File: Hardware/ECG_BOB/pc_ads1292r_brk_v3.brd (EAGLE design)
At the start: 33.9 x 39.9 mm, 64 parts, among them Q1 BSS138, Q2 BSS138, Q3 BSS138, Q4 BSS138, Q5 BSS138, Q6 BSS138, Q7 BSS138

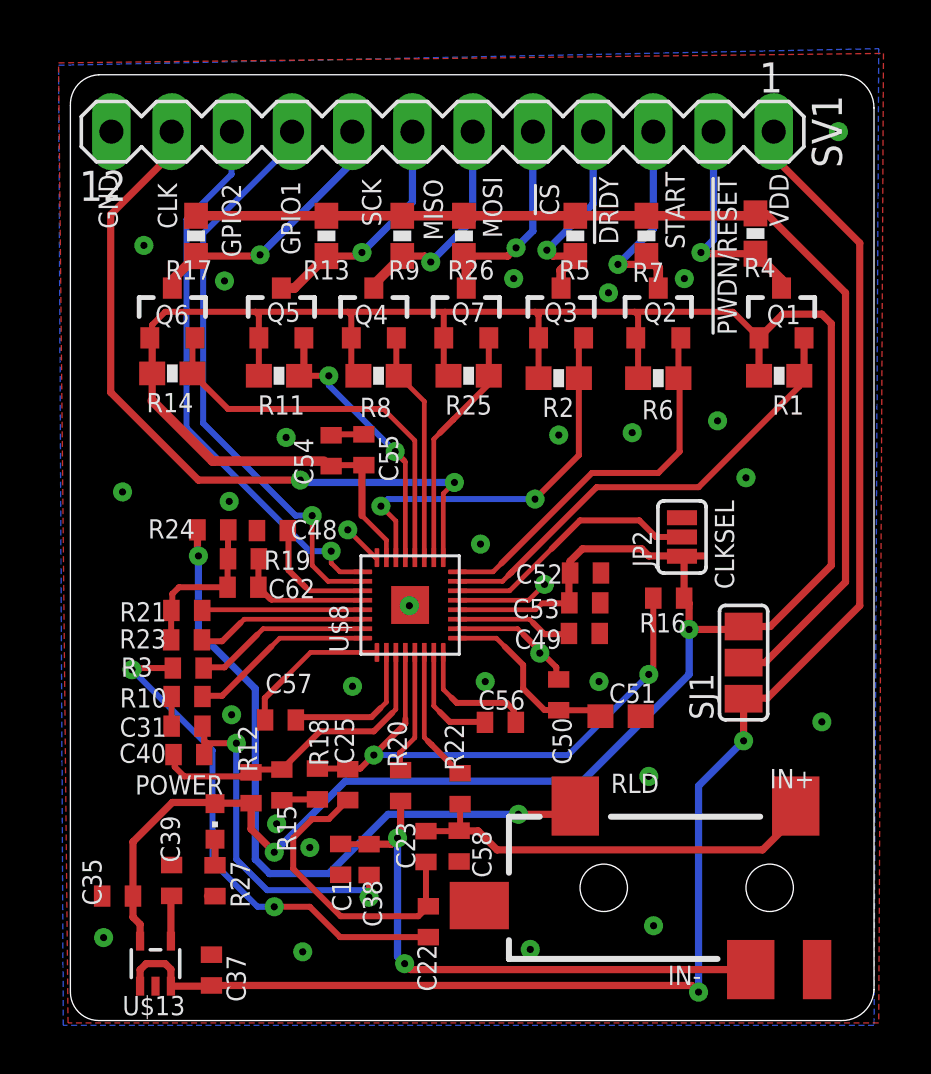
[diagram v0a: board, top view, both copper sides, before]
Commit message: added new design file
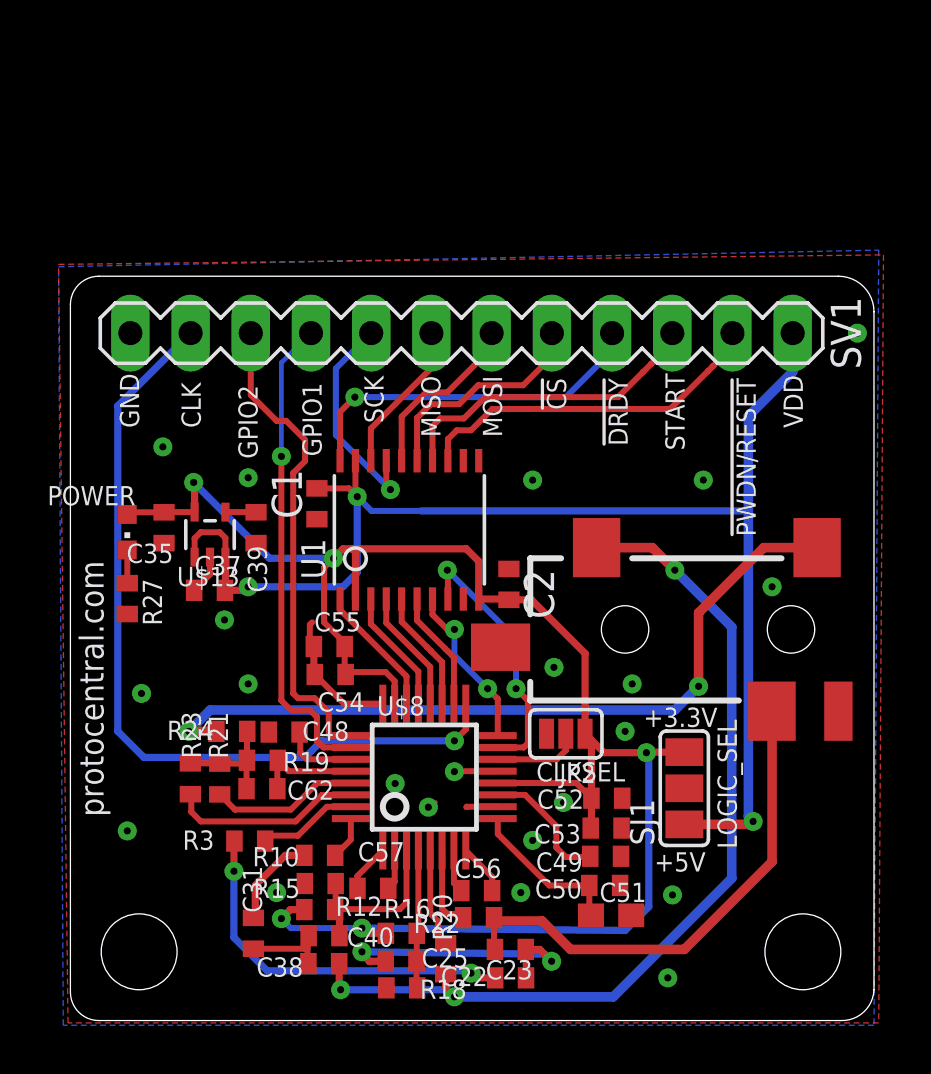
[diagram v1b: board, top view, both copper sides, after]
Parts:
- removed C58: DNP, rcl:C0402
- removed Q1, Q2, Q3, Q4, Q5, Q6, Q7: BSS138, SparkFun:SOT23-3
- removed R1, R11, R13, R14, R17, R2, R25, R26, R4, R5, R6, R7, R8, R9: 10K, SparkFun:0603-RES
- added C2: 100n, rcl:C0402
- added LOGO1: OSHW_LOGO_FILLX0100-NT, ohw-logo:OSHW_FILLX100_NOTEXT
- added U1: (no value), adafruit:TSSOP20
- C1: value (none) -> 100n
- U$8: value (none) -> ADS1292R-TQFP; device circuitects:S-PVQFN-N32 -> circuitects:SQFP-S-5X5-32
- moved U$13 18.2 mm to (5.99, 20.6)
- moved R16 18.1 mm to (14.1, 3.78), turned to 0 degrees
- moved C37 16.0 mm to (5.97, 18.2), turned to 0 degrees
- moved C35 15.7 mm to (4.05, 20.9), turned to 90 degrees
- moved C39 15.3 mm to (7.93, 20.9), turned to 90 degrees
- moved C1 15.0 mm to (10.5, 21.9), turned to 90 degrees
- moved POWER 12.7 mm to (2.50, 20.7)
- moved R27 12.5 mm to (2.50, 17.9)
- moved JP3 10.9 mm to (34.0, 16.6)
- moved JP2 9.64 mm to (21.0, 12.2), turned to 180 degrees
- moved C52 9.54 mm to (22.7, 9.48)
- moved C53 9.54 mm to (22.7, 8.22)
- moved C40 9.53 mm to (10.8, 3.68), turned to 0 degrees
- moved C49 9.44 mm to (22.7, 7.03)
- moved C54 9.44 mm to (11.1, 14.7), turned to 0 degrees
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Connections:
- net !ADS_DRDY: now also U1.1; no longer Q3.2, R2.2
- net !ARD_DRDY: now also U1.20; no longer Q3.3, R5.2
- net +3V3: now also C2.2, U1.10, U1.2; no longer Q1.1, Q2.1, Q3.1, Q4.1, Q5.1, Q6.1, Q7.1, R1.1, R11.1, R14.1, R2.1, R25.1, R6.1, R8.1
- net +5V: now also C1.2, U1.19
- net ADS_PWDN: now also U1.8; no longer Q1.2, R1.2
- net ADS_START: now also U1.7; no longer Q2.2, R6.2
- net ARD_CS0: now also U1.15; no longer Q7.3, R26.2
- net ARD_MISO: now also U1.18; no longer Q5.3, R13.2
- net ARD_MOSI: now also U1.16; no longer Q4.3, R9.2
- net ARD_PWDN: now also U1.13; no longer Q1.3, R4.2
- net ARD_SCK: now also U1.17; no longer Q6.3, R17.2
- net ARD_START: now also U1.14; no longer Q2.3, R7.2
- net GND: now also C1.1, C2.1, U1.11; no longer C1.2, C58.1
- net N$30: now also JP3.TIP; no longer C1.1, JP3.RING
- net N$45: now also JP3.RING; no longer C58.2, JP3.SLEEVE
- net N$51: now also JP3.SLEEVE; no longer JP3.TIP
- net SPI_CS0: now also U1.6; no longer Q7.2, R25.2
- net SPI_MISO: now also U1.3; no longer Q5.2, R11.2
- net SPI_MOSI: now also U1.5; no longer Q4.2, R8.2
- net SPI_SCK: now also U1.4; no longer Q6.2, R14.2
- net VCC: no longer R13.1, R17.1, R26.1, R4.1, R5.1, R7.1, R9.1
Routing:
- net +3V3: track 131.8 -> 76.8 mm, vias 2 -> 5
- net VCC: track 46.7 -> 0.00 mm
- net N$32: track 24.1 -> 5.84 mm, vias 2 -> 0
- net N$30: track 24.3 -> 38.7 mm, vias 2 -> 3
- net SPI_SCK: track 17.0 -> 5.18 mm
- net !ADS_DRDY: track 16.7 -> 5.57 mm, vias 2 -> 0
- net N$29: track 14.8 -> 4.57 mm, vias 2 -> 0
- net ADS_START: track 16.3 -> 7.08 mm, vias 0 -> 2
- net ADS_PWDN: track 20.1 -> 11.3 mm, vias 0 -> 2
- net +5V: track 66.5 -> 58.2 mm, vias 2 -> 3
- net N$104: track 11.0 -> 3.73 mm
- net SPI_MISO: track 11.9 -> 5.24 mm, vias 2 -> 0
- net !ARD_DRDY: track 8.71 -> 15.3 mm
- net N$31: track 13.9 -> 7.67 mm
- net SPI_CS0: track 11.1 -> 5.06 mm
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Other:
- board size 33.9 x 39.9 mm -> 33.9 x 31.4 mm
- board text added: "+3.3V"
- board text added: "+5V"
- board text added: "ADS1292R Breakout - v3"
- board text added: "LOGIC_SEL"
- board text added: "pc_ads1292r_brk_v3"
- board text added: "protocentral.com"
- board text removed: "ADS1292R Breakout"
- board text removed: "IN+"
- board text removed: "IN-"
- board text removed: "RLD"
